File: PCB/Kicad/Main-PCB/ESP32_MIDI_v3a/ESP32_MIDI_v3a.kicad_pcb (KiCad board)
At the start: 2 copper layers, 189 x 27 mm, 26 parts

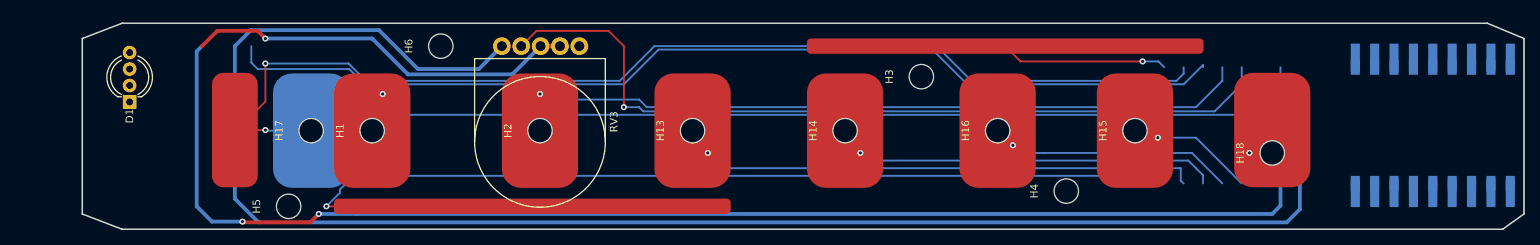
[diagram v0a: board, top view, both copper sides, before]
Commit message: Jan 10 commit - up to v4
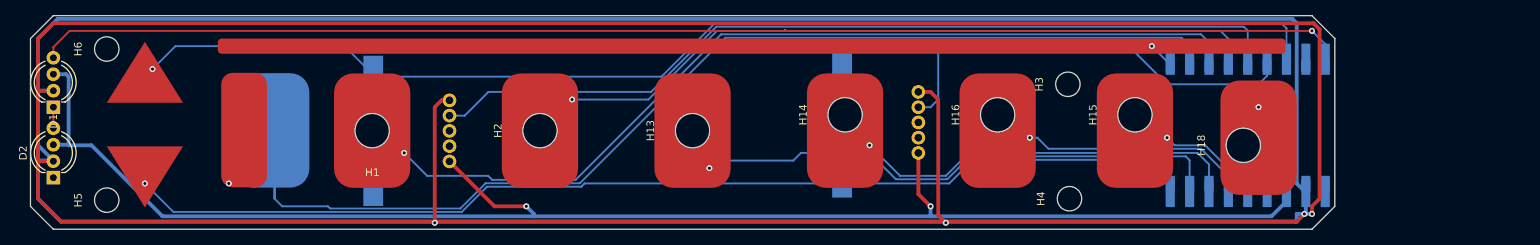
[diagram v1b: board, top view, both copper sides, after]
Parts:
- removed H17: MountingHole, MountingHole:MountingHole_3.2mm_M3
- removed RV3: R_Potentiometer_Dual, ih_kicad:potentiometer_wheel_16mm
- added D2: WS2812B, LED_THT:LED_D5.0mm-4_RGB_Wide_Pins, F.Cu at (39.0, 104.2)
- added RV2: R_Potentiometer_Dual, ih_kicad:potentiometer_wheel_10mm_SMD-shield, B.Cu at (83.4, 98.1)
- added RV4: R_Potentiometer_Dual, ih_kicad:potentiometer_wheel_10mm_SMD-shield, B.Cu at (144.9, 97.0)
- added TP12: TestPoint, ih_kicad:recorder-touchpad-alt-up, F.Cu at (51.0, 90.4)
- H1, H13, H14, H15, H16, H18, H2: footprint MountingHole:MountingHole_3.2mm_M3 -> MountingHole:MountingHole_4.5mm
- H3, H4, H5, H6: footprint MountingHole:MountingHole_3.2mm_M3 -> MountingHole:MountingHole_3.2mm_M3_ISO14580
- TP8: footprint ih_kicad:recorder-touchtrack -> ih_kicad:recorder-touchpad-alt-up
- TP9: footprint ih_kicad:recorder-touchtrack -> ih_kicad:recorder-touchtrack_120mm
- moved TP8 114.1 mm to (51.0, 104.1)
- moved H6 43.8 mm to (46.0, 87.4)
- moved TP9 35.6 mm to (130.6, 87.0), turned to 0 degrees
- moved U2 24.3 mm to (195.6, 97.4)
- moved H5 23.9 mm to (46.0, 107.2)
- moved H3 19.2 mm to (172.0, 92.0)
- moved D1 10.0 mm to (39.0, 95.0)
- moved TP1 5.23 mm to (67.6, 98.0)
- moved H18 3.92 mm to (195.0, 100.0)
- moved H14 2.08 mm to (142.8, 96.0)
- moved H15 2.08 mm to (180.8, 96.0)
- moved H16 2.08 mm to (162.8, 96.0)
- moved TP10 2.05 mm to (197.0, 99.0)
- moved TP11 1.21 mm to (64.0, 98.0)
- moved H4 1.08 mm to (172.2, 107.0)
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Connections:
- D1 pad 1: +3.3V -> Net-(D1-DOUT)
- D1 pad 2: unconnected-(D1-DOUT-Pad2) -> GND
- D1 pad 3: GND -> +3.3V
- D1 pad 4: /D2 -> /SCL
- TP8 pad 1: /A6 -> /A5
- TP9 pad 1: /A5 -> /A6
- U2 pad 16: /D2 -> /A10
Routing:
- net GND: track 204.2 -> 820.4 mm, vias 0 -> 4
- net /SCL: track 0.00 -> 172.8 mm, vias 0 -> 1
- net /A10: track 0.00 -> 161.0 mm, vias 0 -> 1
- net /D2: track 143.2 -> 0.00 mm
- net /D1: track 0.00 -> 57.3 mm
- net +3.3V: track 219.7 -> 203.0 mm, vias 3 -> 2
- net /A6: track 22.0 -> 5.76 mm
- net /A7: track 147.3 -> 157.5 mm, vias 2 -> 1
- net /A8: track 113.2 -> 121.3 mm
- net /D0: track 108.1 -> 114.5 mm, vias 1 -> 0
- net /A4: track 66.8 -> 72.9 mm
- net /A3: track 49.0 -> 54.3 mm
- net /A9: track 97.1 -> 101.0 mm
- net Net-(D1-DOUT): track 0.00 -> 3.76 mm
- net /A5: track 139.2 -> 142.5 mm
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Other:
- board size 189 x 27 mm -> 171 x 28 mm
- board text added: "Robin v3a Jan24 Ian Hattwick"
- board text added: "Somerville, MA Jan24"
- board text added: "long"
